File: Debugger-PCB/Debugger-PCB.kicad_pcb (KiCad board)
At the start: 2 copper layers, 72.1 x 49.7 mm, 67 parts, among them J1 Conn_01x04, J2 USB_C_Receptacle_USB2.0, J3 Conn_01x04, J4 Conn_01x02, Q1 S8050, SW1 SW_Push, SW2 SW_Push, SW3 SW_Push, U1 HX9193, U2 CH340E, U3 HX9193, U4 TJA1051T-3, U5 STM32F407VETx, U6 REF3030, U7 XPT2046TS, U8 W25Q32JVSS, Y1 12M

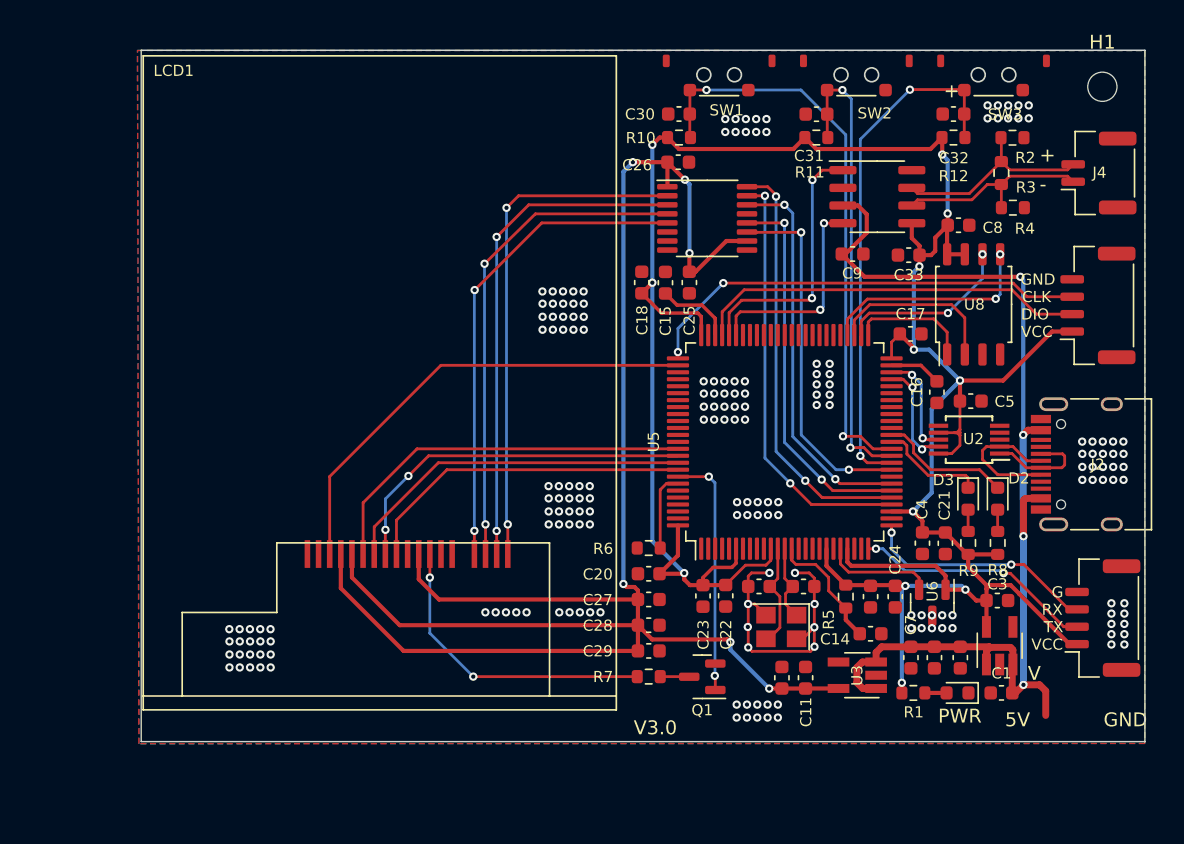
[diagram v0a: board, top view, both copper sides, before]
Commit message: temp.change the PCB.And change the code.
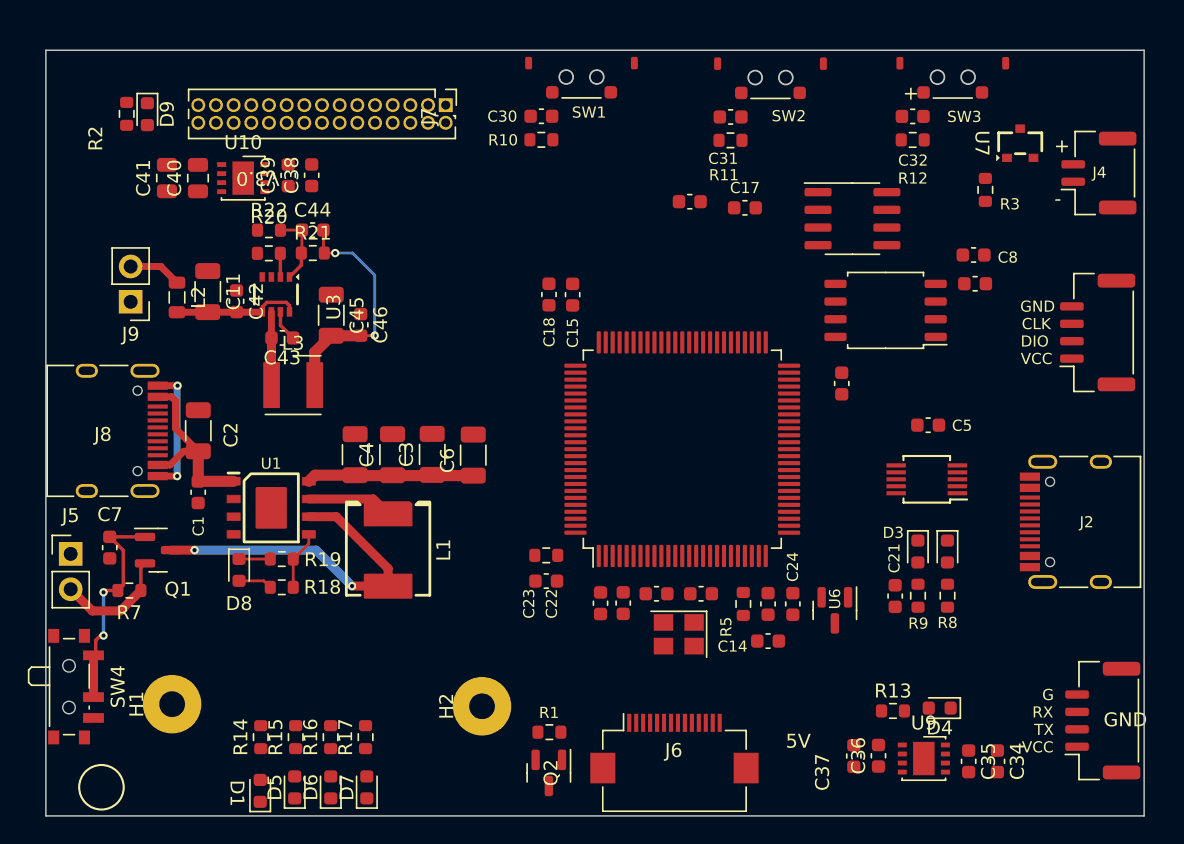
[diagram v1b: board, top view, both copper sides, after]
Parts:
- removed C25, C26, C27, C28, C29: 100n, Capacitor_SMD:C_0603_1608Metric
- removed LCD1: 1.8inch-TFT-LCD, debugger:TFT-LCD1.8inch
- removed R4: 10k, Resistor_SMD:R_0603_1608Metric
- added C34: 4.7u, Capacitor_SMD:C_0603_1608Metric, F.Cu at (178.5, 134.7)
- added C35: 100n, Capacitor_SMD:C_0603_1608Metric, F.Cu at (176.4, 134.7)
- added C36: 4.7u, Capacitor_SMD:C_0603_1608Metric, F.Cu at (169.9, 134.3)
- added C37: 100n, Capacitor_SMD:C_0603_1608Metric, F.Cu at (168.2, 134.3)
- added C38: 4.7u, Capacitor_SMD:C_0603_1608Metric, F.Cu at (129.2, 92.5)
- added C39: 100n, Capacitor_SMD:C_0603_1608Metric, F.Cu at (127.5, 92.6)
- added C40: 4.7u, Capacitor_SMD:C_0805_2012Metric, F.Cu at (121.0, 92.8)
- added C41: 100n, Capacitor_SMD:C_0805_2012Metric, F.Cu at (118.8, 92.8)
- added C42: 100n, Capacitor_SMD:C_0603_1608Metric, F.Cu at (123.8, 101.6)
- added C43: 103, Capacitor_SMD:C_0603_1608Metric, F.Cu at (127.1, 104.2)
- added C44: 101, Capacitor_SMD:C_0603_1608Metric, F.Cu at (129.3, 96.5)
- added C45: 22uf 0603, Capacitor_SMD:C_1206_3216Metric, F.Cu at (130.6, 102.6)
- added C46: 104, Capacitor_SMD:C_0603_1608Metric, F.Cu at (132.7, 103.3)
- added D4: LED, LED_SMD:LED_0603_1608Metric, F.Cu at (174.3, 130.8)
- added D5: , LED_SMD:LED_0603_1608Metric, F.Cu at (128.0, 136.5)
- added D6: , LED_SMD:LED_0603_1608Metric, F.Cu at (130.6, 136.5)
- added D7: , LED_SMD:LED_0603_1608Metric, F.Cu at (133.2, 136.5)
- added D8: , LED_SMD:LED_0603_1608Metric, F.Cu at (124.0, 120.9)
- added D9: LED, LED_SMD:LED_0603_1608Metric, F.Cu at (117.4, 88.2)
- added H2: MountingHole, ic:mo, F.Cu at (141.5, 130.7)
- added J5: Conn_01x02, Connector_PinHeader_2.54mm:PinHeader_1x02_P2.54mm_Vertical, F.Cu at (111.9, 119.8)
- added J6: Conn_01x14, Connector_FFC-FPC:Hirose_FH12-14S-0.5SH_1x14-1MP_P0.50mm_Horizontal, F.Cu at (155.3, 133.8)
- added J7: axt430124, Connector_PinHeader_1.27mm:PinHeader_2x15_P1.27mm_Vertical, F.Cu at (138.8, 87.5)
- added J8: USB_C_Receptacle_USB2.0, Connector_USB:USB_C_Receptacle_HRO_TYPE-C-31-M-12, F.Cu at (114.1, 110.9)
- added J9: Conn_01x02, Connector_PinHeader_2.54mm:PinHeader_1x02_P2.54mm_Vertical, F.Cu at (116.2, 101.6)
- added L1: 1u, PCM_008_GN_POWER-CHOKE_SMD:MC-0630, F.Cu at (134.7, 119.5)
- added L2: 600r, Inductor_SMD:L_0805_2012Metric, F.Cu at (119.5, 101.3)
- added L3: 2.2uh, Inductor_SMD_Wurth:L_Wurth_WE-LQSH-4020, F.Cu at (127.9, 107.6)
- added Q2: SI2301, Package_TO_SOT_SMD:SOT-23, F.Cu at (146.3, 135.5)
- added R13: 1K, Resistor_SMD:R_0603_1608Metric, F.Cu at (171.0, 131.0)
- added R14: 10k, Resistor_SMD:R_0603_1608Metric, F.Cu at (125.6, 132.9)
- added R15: 10k, Resistor_SMD:R_0603_1608Metric, F.Cu at (128.1, 132.9)
- added R16: 10k, Resistor_SMD:R_0603_1608Metric, F.Cu at (130.6, 132.9)
- added R17: 10k, Resistor_SMD:R_0603_1608Metric, F.Cu at (133.1, 132.9)
- added R18: 10k, Resistor_SMD:R_0603_1608Metric, F.Cu at (127.1, 122.2)
- added R19: 10k, Resistor_SMD:R_0603_1608Metric, F.Cu at (127.1, 120.1)
- added R20: 200K, Resistor_SMD:R_0603_1608Metric, F.Cu at (126.1, 98.2)
- added R21: 220K, Resistor_SMD:R_0603_1608Metric, F.Cu at (129.3, 98.1)
- added R22: 30k, Resistor_SMD:R_0603_1608Metric, F.Cu at (126.2, 96.5)
- added SW4: SW_SPDT, Button_Switch_SMD:SW_SPDT_PCM12, F.Cu at (112.1, 129.3)
- added U10: ~, Package_DFN_QFN:DFN-8-1EP_3x3mm_P0.65mm_EP1.55x2.4mm, F.Cu at (124.3, 92.8)
- added U9: ~, Package_DFN_QFN:DFN-8-1EP_3x3mm_P0.65mm_EP1.55x2.4mm, F.Cu at (173.2, 134.5)
- C1: value 10u -> 100n
- C10, C3: value 100n -> 22u; footprint Capacitor_SMD:C_0603_1608Metric -> Capacitor_SMD:C_1206_3216Metric
- C11: value 10u -> 106 1206; footprint Capacitor_SMD:C_0603_1608Metric -> Capacitor_SMD:C_1206_3216Metric
- C2: value 100n -> 10u; footprint Capacitor_SMD:C_0603_1608Metric -> Capacitor_SMD:C_1206_3216Metric
- C4, C6: value 10u -> 22u; footprint Capacitor_SMD:C_0603_1608Metric -> Capacitor_SMD:C_1206_3216Metric
- D1: value LED -> (none)
- H1: value mountinghole -> MountingHole; footprint MountingHole:MountingHole_2.1mm -> ic:mo
- Q1: value S8050 -> AO3407
- R1: value 1k -> 10K
- R2: value 10k -> 1K
- R7: value R -> 10k
- U1: value HX9193 -> IP5306; footprint Package_TO_SOT_SMD:SOT-23-5_HandSoldering -> PCM_004_GN_MIDDLE-SEMI_SMD:SOP-8EP_3949
- U3: value HX9193 -> SY8303; footprint Package_TO_SOT_SMD:SOT-23-5_HandSoldering -> PCM_003_GN_SMALL-SEMI_SMD:SOT-23-8
- U7: value XPT2046TS -> pesd1can; footprint debugger:TSSOP-16_4.4x5mm_P0.65mm -> PCM_003_GN_SMALL-SEMI_SMD:SOT-23
- moved H1 80.2 mm to (119.2, 130.6), turned to 90 degrees
- moved R2 63.7 mm to (115.9, 88.1), turned to -90 degrees
- moved C1 59.5 mm to (121.1, 115.3), turned to 90 degrees
- moved C7 58.1 mm to (114.7, 119.3)
- moved C2 57.1 mm to (121.1, 110.9)
- moved U1 53.3 mm to (126.3, 116.5), turned to 0 degrees
- moved C11 51.1 mm to (121.8, 100.9), turned to -90 degrees
- moved D1 50.6 mm to (125.5, 136.8), turned to 90 degrees
- moved U3 49.9 mm to (126.7, 101.1), turned to 90 degrees
- moved C3 41.9 mm to (137.9, 112.6), turned to 90 degrees
- moved Q1 40.2 mm to (118.2, 119.5), turned to 0 degrees
- moved C4 38.6 mm to (135.0, 112.6), turned to 90 degrees
- moved R7 37.8 mm to (116.1, 122.4)
- moved C6 36.2 mm to (140.8, 112.7), turned to 90 degrees
- moved C10 34.6 mm to (132.3, 112.6)
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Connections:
- net Net-(U5-NRST) renamed /MCU/RESET
- C1 pad 1: +5V -> GND
- C1 pad 2: GND -> BATE_5V
- C10 pad 1: LCD_3V3 -> +5V
- C10 pad 2: GND -> GND1
- C11 pad 1: LCD_3V3 -> GND
- C11 pad 2: GND -> Net-(U3-EN)
- C2 pad 1: +5V -> GND
- C2 pad 2: GND -> BATE_5V
- C3 pad 1: VCC -> +5V
- C3 pad 2: GND -> GND1
- C4 pad 1: VCC -> +5V
- C4 pad 2: GND -> GND1
- C6 pad 2: GND -> GND1
- C7 pad 1: +5V -> G
- D1 pad 1: GND -> Net-(D1-Cathode)
- D1 pad 2: Net-(D1-A) -> Net-(D1-Anode)
- Q1 pad 1: /MCU/LCD_LED -> G
- Q1 pad 2: GND -> /Power&Port/VBAT+
- Q1 pad 3: Net-(Q1-C) -> /Power&Port/VBAT
- R1 pad 1: VCC -> /MCU/LCD_LED
- R1 pad 2: Net-(D1-A) -> GND
- R2 pad 1: GND -> VCC
- R2 pad 2: /Power&Port/CAN+ -> Net-(D9-A)
- R7 pad 1: /TFT/LED- -> G
- R7 pad 2: Net-(Q1-C) -> /Power&Port/VBAT+
- U1 pad 1: +5V -> BATE_5V
- U1 pad 2: GND -> Net-(U1-LED1)
- U1 pad 3: +5V -> Net-(U1-LED2)
- U1 pad 4: unconnected-(U1-NC-Pad4) -> Net-(D1-Cathode)
- U1 pad 5: VCC -> Net-(U1-KEY)
- U3 pad 1: +5V -> Net-(U3-FB)
- U3 pad 2: GND -> Net-(U3-FS)
- U3 pad 3: +5V -> GND
- U3 pad 4: unconnected-(U3-NC-Pad4) -> GND
- U3 pad 5: LCD_3V3 -> Net-(U3-EN)
- U5 pad 15: unconnected-(U5-PC0-Pad15) -> /MCU/LCD_CS0
- U5 pad 16: unconnected-(U5-PC1-Pad16) -> /MCU/ADC1_IN11
- U5 pad 17: unconnected-(U5-PC2-Pad17) -> /MCU/ADC1_IN12
- U5 pad 18: unconnected-(U5-PC3-Pad18) -> /MCU/ADC1_IN13
- U5 pad 23: unconnected-(U5-PA0-Pad23) -> /MCU/ADC1_IN0
- U5 pad 24: unconnected-(U5-PA1-Pad24) -> /MCU/ADC1_IN1
- U5 pad 33: unconnected-(U5-PC4-Pad33) -> /MCU/ADC1_IN14
- U5 pad 40: unconnected-(U5-PE9-Pad40) -> /MCU/TIM1_CH1
- U5 pad 42: unconnected-(U5-PE11-Pad42) -> /MCU/TIM1_CH2
- U5 pad 56: unconnected-(U5-PD9-Pad56) -> /MCU/I2C3_SDA
- U5 pad 59: unconnected-(U5-PD12-Pad59) -> /MCU/TIM4_CH2
- U5 pad 60: unconnected-(U5-PD13-Pad60) -> /MCU/TIM4_CH1
- U5 pad 63: unconnected-(U5-PC6-Pad63) -> /MCU/TIM3_CH1
- U5 pad 64: unconnected-(U5-PC7-Pad64) -> /MCU/TIM3_CH2
- U5 pad 67: unconnected-(U5-PA8-Pad67) -> /MCU/I2C3_SCL
- U5 pad 68: unconnected-(U5-PA9-Pad68) -> /MCU/KEY5
- U5 pad 69: unconnected-(U5-PA10-Pad69) -> /MCU/KEY4
- U5 pad 95: unconnected-(U5-PB8-Pad95) -> /MCU/LCD_CS
- U5 pad 96: unconnected-(U5-PB9-Pad96) -> /MCU/LCD_DC
- U7 pad 1: LCD_3V3 -> /Power&Port/CAN+
- U7 pad 2: /TFT/T_XP -> /Power&Port/CAN-
- U7 pad 3: /TFT/T_YP -> GND
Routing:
- net VCC: track 196.2 -> 3.81 mm, vias 12 -> 0
- net LCD_3V3: track 138.2 -> 0.00 mm, vias 6 -> 0
- net +5V: track 78.0 -> 29.6 mm, vias 4 -> 2
- net /Key&LED/KEY1: track 41.6 -> 0.00 mm, vias 2 -> 0
- net /Key&LED/KEY3: track 37.6 -> 0.00 mm, vias 2 -> 0
- net /TFT/T_XP: track 36.8 -> 0.00 mm, vias 2 -> 0
- net /TFT/T_YP: track 36.0 -> 0.00 mm, vias 2 -> 0
- net /TFT/T_XM: track 35.5 -> 0.00 mm, vias 2 -> 0
- net /TFT/T_YM: track 34.8 -> 0.00 mm, vias 2 -> 0
- net /MCU/LCD_CS: track 33.9 -> 0.00 mm
- net /Key&LED/KEY2: track 33.7 -> 0.00 mm, vias 2 -> 0
- net /MCU/SWCLK: track 32.2 -> 0.00 mm, vias 2 -> 0
- net /MCU/TOUCH_CS: track 30.6 -> 0.00 mm, vias 2 -> 0
- net /MCU/TOUCH_CLK: track 30.4 -> 0.00 mm, vias 2 -> 0
- net /MCU/SWDIO: track 28.2 -> 0.00 mm
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- removed copper zone on B.Cu, net GND
- removed copper zone on F.Cu, net GND
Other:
- board size 72.1 x 49.7 mm -> 78.9 x 55 mm
- board text removed: "V"
